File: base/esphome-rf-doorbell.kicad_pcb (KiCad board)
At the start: 2 copper layers, 65 x 54.7 mm, 100 parts, among them J1 B4B-XH, J2 CONUFL001-SMD-T, J3 Conn_01x01, J4 Conn_01x01, SW1 Boot, U1 BQ25628E, U2 RFM69W, U3 TPS7A2033, U4 MAX17261xxTD, U5 TPS629206DRLR, U6 G3VM-31DR, U7 ESP32-S2-MINI-2, U8 G3VM-63ER, U9 TLP2391

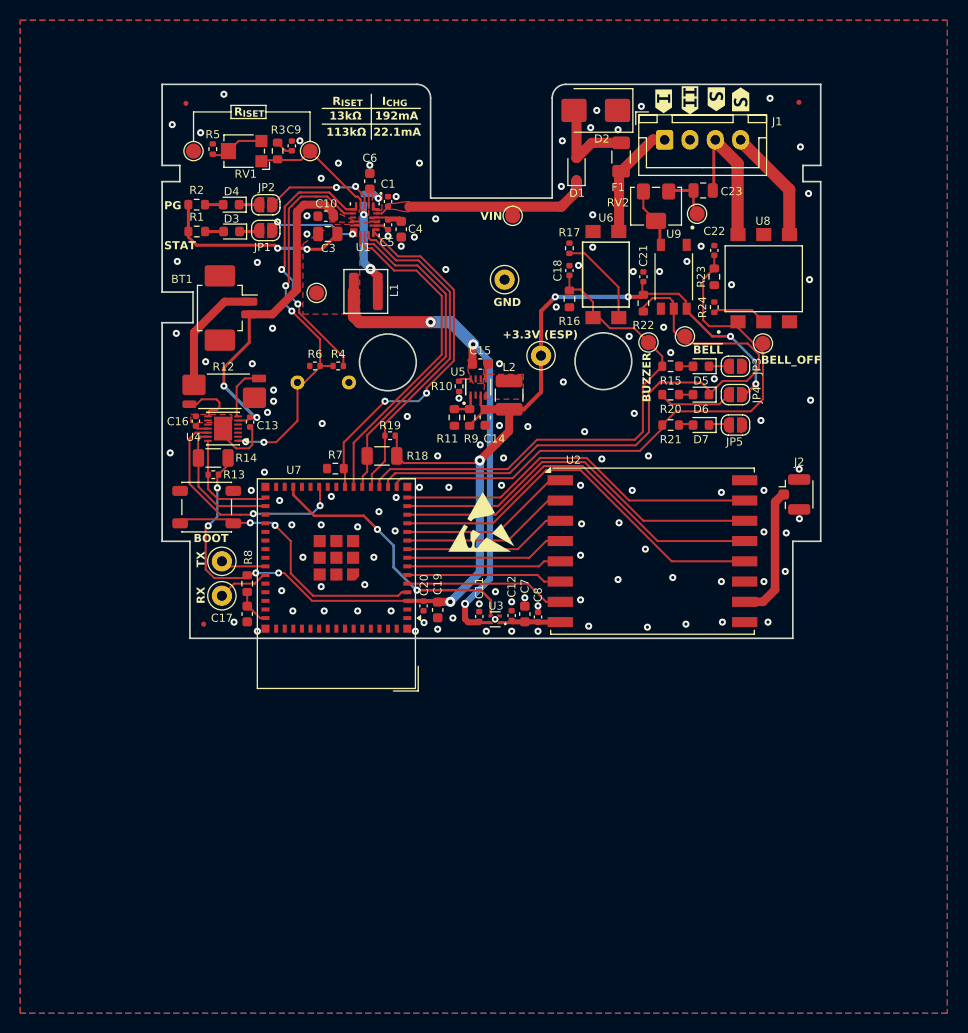
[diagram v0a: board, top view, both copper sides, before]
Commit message: Base board Rev3
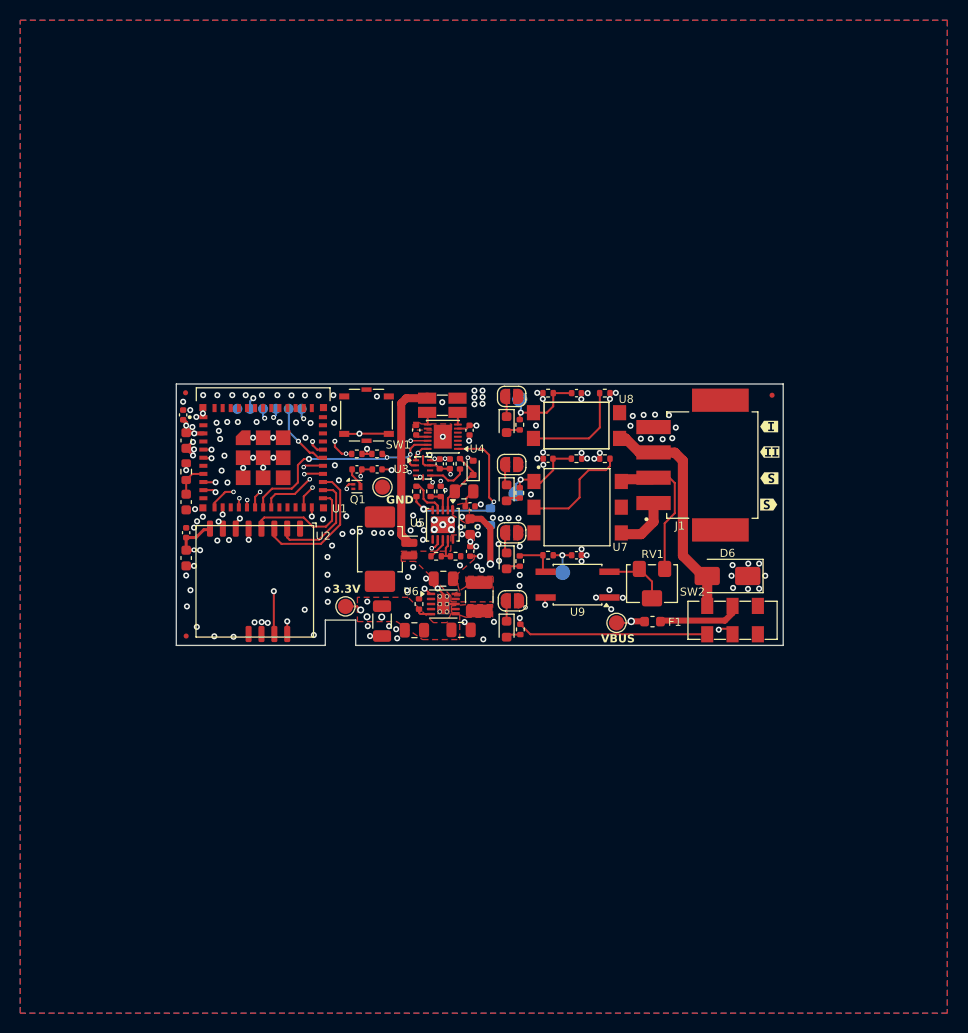
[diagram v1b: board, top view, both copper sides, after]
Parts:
- removed the C1 at (130.3, 77.9)
- removed the C2 at (127.9, 77.7)
- removed C21: 0.1uF, Capacitor_SMD:C_0402_1005Metric
- removed C23: 1uF 50V, Capacitor_SMD:C_0805_2012Metric
- removed the C3 at (124.3, 81.1)
- removed the C4 at (131.6, 80.6)
- removed the C5 at (130.3, 80.2)
- removed the D3 at (114.9, 80.8)
- removed the D4 at (114.8, 78.2)
- removed J3, J4: Conn_01x01, TestPoint:TestPoint_Keystone_5000-5004_Miniature
- removed the JP1 at (118.2, 80.8)
- removed the JP2 at (118.2, 78.2)
- removed L2: 2.2uH, Inductor_SMD:L_1210_3225Metric
- removed the R1 at (111.4, 80.8)
- removed the R10 at (137.3, 96.1)
- removed the R2 at (111.4, 78.2)
- removed the R20 at (158.2, 96.9)
- removed the R21 at (158.2, 99.9)
- removed the R4 at (125.4, 94.1)
- removed the REF** at (139.5, 109.5)
- removed the REF** at (117.4, 72.1)
- removed the RV1 at (116.0, 72.9)
- removed the TP1 at (122.6, 72.9)
- removed TP11: TestPoint, TestPoint:TestPoint_Pad_D1.5mm
- removed the TP4 at (123.2, 86.9)
- removed the TP5 at (111.1, 72.9)
- removed the U7 at (125.2, 115.6)
- removed kibuzzard-691E1EB0: G***, kibuzzard-691E1EB0
- removed kibuzzard-691E1EB7: G***, kibuzzard-691E1EB7
- removed kibuzzard-691E1ECB: G***, kibuzzard-691E1ECB
- removed kibuzzard-691E1ED6: G***, kibuzzard-691E1ED6
- added C16: 1uF, Capacitor_SMD:C_0402_1005Metric, F.Cu at (138.4, 112.4)
- added C19: 1uF, Capacitor_SMD:C_0402_1005Metric, F.Cu at (148.9, 112.8)
- added C8: 47uF, Capacitor_SMD:C_0805_2012Metric, F.Cu at (132.9, 120.2)
- added D5: Red, LED_SMD:LED_0603_1608Metric, F.Cu at (142.0, 120.1)
- added JP4: SolderJumper_2_Open, Jumper:SolderJumper-2_P1.3mm_Open_RoundedPad1.0x1.5mm, F.Cu at (142.6, 117.3)
- added Q1: PMZB390UNE, Package_DFN_QFN:Diodes_DFN1006-3, F.Cu at (127.2, 106.0)
- added R12: 1.27M, Resistor_SMD:R_0402_1005Metric, F.Cu at (137.0, 112.9)
- added R16: 1k, Resistor_SMD:R_0402_1005Metric, F.Cu at (143.3, 106.6)
- added R17: 1k, Resistor_SMD:R_0402_1005Metric, F.Cu at (143.3, 113.4)
- added R18: 1k, Resistor_SMD:R_0402_1005Metric, F.Cu at (143.4, 120.1)
- added R8: 47k, Resistor_SMD:R_0402_1005Metric, F.Cu at (134.5, 106.5)
- added REF**: KiCad-Logo2_6mm_SilkScreen, Symbol:KiCad-Logo2_6mm_SilkScreen, B.Cu at (118.7, 113.4)
- added SW2: CL-SB-22A-11T, lib:CL-SB-22A, F.Cu at (164.3, 119.2)
- added U6: TPS63900, Package_SON:WSON-10-1EP_2.5x2.5mm_P0.5mm_EP1.2x2mm_ThermalVias, F.Cu at (135.8, 117.6)
- added kibuzzard-696E5F1B: G***, kibuzzard-696E5F1B, F.Cu at (168.0, 102.6)
- added kibuzzard-696E5F26: G***, kibuzzard-696E5F26, F.Cu at (167.9, 100.1)
- added kibuzzard-696E5F32: G***, kibuzzard-696E5F32, F.Cu at (167.9, 105.2)
- added kibuzzard-696E5F3B: G***, kibuzzard-696E5F3B, F.Cu at (167.9, 107.8)
- C10: value 10uF 10V -> 47uF; footprint Capacitor_SMD:C_0603_1608Metric -> Capacitor_SMD:C_0805_2012Metric
- C12: value 1uF -> 47uF; footprint Capacitor_SMD:C_0402_1005Metric -> Capacitor_SMD:C_0805_2012Metric
- C14: value 22uF 6.3V -> 1uF 25V; footprint Capacitor_SMD:C_0603_1608Metric -> Capacitor_SMD:C_0402_1005Metric
- C15: value 4.7uF -> 10uF 25V
- C6: value 4.7uF -> 100uF; footprint Capacitor_SMD:C_0603_1608Metric -> Capacitor_SMD:C_1206_3216Metric
- C7: renamed from C16; value 47nF -> 0.47uF
- C9: value 330nF -> 0.1uF
- D1: value PMEG2005EJ-QX -> BAS70; footprint Diode_SMD:D_SOD-323F -> Diode_SMD:D_SOD-523
- D3: renamed from D7; value Red -> Blue
- D6: renamed from D2; value SMBJ15CA -> SMAJ15CA; footprint Diode_SMD:D_SMB -> Diode_SMD:D_SMA
- F1: value 250mA -> 80mA; footprint Fuse:Fuse_1206_3216Metric -> Fuse:Fuse_0603_1608Metric
- J1: value B4B-XH -> PTSM 0,5/ 4-2,5-H SMD R24; footprint Connector_JST:JST_XH_B4B-XH-A_1x04_P2.50mm_Vertical -> lib:PHOENIX_1702474
- J2: value CONUFL001-SMD-T -> Conn_01x06; footprint Connector_Coaxial:U.FL_Hirose_U.FL-R-SMT-1_Vertical -> lib:Connector_PogoClamp_1.27mm; moved to B.Cu
- L1: value 1.5uH -> 2.2uH; footprint Inductor_SMD:L_Wuerth_MAPI-4020 -> Inductor_SMD:L_1210_3225Metric
- R10: renamed from R12; value 25m -> 15m; footprint Resistor_SMD:R_Shunt_Vishay_WSK2512_6332Metric_T1.19mm -> lib:R_Shunt_D1WRL1206
- R11: value 137k -> 30k; footprint Resistor_SMD:R_0603_1608Metric -> Resistor_SMD:R_0402_1005Metric
- R13: value 4.7k -> 120k
- R14: value 4.7k -> 820k; footprint Resistor_SMD:R_1206_3216Metric -> Resistor_SMD:R_0805_2012Metric
- R15: footprint Resistor_SMD:R_0603_1608Metric -> Resistor_SMD:R_0402_1005Metric
- R19: renamed from R16; value 10k -> 100k; footprint Resistor_SMD:R_0603_1608Metric -> Resistor_SMD:R_0402_1005Metric
- R2: renamed from R18; value 4.7k -> 16.9k; footprint Resistor_SMD:R_1206_3216Metric -> Resistor_SMD:R_0402_1005Metric
- R20: renamed from R22; footprint Resistor_SMD:R_0603_1608Metric -> Resistor_SMD:R_0402_1005Metric
- R21: renamed from R23; value 10k -> 100k; footprint Resistor_SMD:R_0603_1608Metric -> Resistor_SMD:R_0402_1005Metric
- R3: value 1.2k -> 100k 0.1%; footprint Resistor_SMD:R_0603_1608Metric -> Capacitor_SMD:C_0402_1005Metric
- R4: renamed from R19; value 4.7k -> 16.9k
- R5: value 13k -> 1M 0.1%; footprint Resistor_SMD:R_0402_1005Metric -> Capacitor_SMD:C_0402_1005Metric
- R6: value 30.1k -> 10k
- R7: value 10k -> 16.2k; footprint Resistor_SMD:R_0603_1608Metric -> Resistor_SMD:R_0402_1005Metric
- R9: value 619k -> 499k; footprint Resistor_SMD:R_0603_1608Metric -> Resistor_SMD:R_0402_1005Metric
- SW1: value Boot -> Flash; footprint Button_Switch_SMD:SW_SPST_PTS647_Sx50 -> Button_Switch_SMD:SW_SPST_Panasonic_EVQPL_3PL_5PL_PT_A08
- TH1: footprint Resistor_THT:R_Axial_DIN0204_L3.6mm_D1.6mm_P5.08mm_Vertical -> Resistor_SMD:R_0603_1608Metric
- TP1: renamed from TP2; footprint TestPoint:TestPoint_Keystone_5000-5004_Miniature -> TestPoint:TestPoint_Pad_D1.5mm
- TP2: renamed from TP7; footprint TestPoint:TestPoint_Keystone_5000-5004_Miniature -> TestPoint:TestPoint_Pad_D1.5mm
- TP4: renamed from TP8; moved to B.Cu
- TP5: renamed from TP9; moved to B.Cu
- TP6: renamed from TP10; moved to B.Cu
- U1: value BQ25628E -> ESP32-C6-MINI-1; footprint lib:WQFN-HR18__RYK_TEX -> lib:XCVR_ESP32-C6-MINI-1U-N4
- U2: value RFM69W -> Wio-SX1262; footprint RF_Module:HOPERF_RFM69HW -> lib:Wio-SX1262 PCB Package
- U3: value TPS7A2033 -> ISL23315; footprint Package_SON:Texas_X2SON-4_1x1mm_P0.65mm -> lib:L10_2P1X1P6A_INR
- U4: value MAX17261xxTD -> MAX17260
- U5: value TPS629206DRLR -> LTC4079; footprint lib:SOT5X3-8_DRL_TEX -> Package_DFN_QFN:DFN-10-1EP_3x3mm_P0.5mm_EP1.65x2.38mm
- U9: value TLP2391 -> LTV-354T; footprint lib:OPTO_TLP2367_TPR_E -> Package_SO:SO-4_4.4x3.6mm_P2.54mm
- moved J2 52.5 mm to (118.6, 98.3), turned to 90 degrees
- moved D6 47.8 mm to (163.8, 114.8)
- moved F1 46.0 mm to (156.4, 119.3), turned to 180 degrees
- moved C6 43.4 mm to (129.7, 119.3), turned to -90 degrees
- moved TP3 41.5 mm to (152.8, 119.5)
- moved J1 38.5 mm to (166.8, 109.2), turned to 90 degrees
- moved C10 37.6 mm to (135.8, 115.1), turned to 180 degrees
- moved RV1 37.3 mm to (156.3, 115.6)
- moved REF** 36.1 mm to (118.7, 107.0)
- moved C4 35.7 mm to (110.4, 110.6)
- moved R5 35.5 mm to (129.2, 104.3), turned to 180 degrees
- moved C9 34.6 mm to (135.4, 103.8), turned to 90 degrees
- moved C5 33.9 mm to (110.4, 113.1), turned to -90 degrees
- moved U2 33.5 mm to (122.9, 109.9), turned to 180 degrees
- moved R3 32.4 mm to (127.2, 104.3), turned to 180 degrees
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- renumbered C20 to C1, C22 to C17, C19 to C2, C17 to C3, C8 to C4, C7 to C5, D5 to D2, D6 to D4, FID3 to FID2, FID2 to FID3, JP3 to JP1, JP5 to JP2, JP4 to JP3, R8 to R1, R17 to R22, R24 to R23, RV2 to RV1, TP6 to TP3, U8 to U7, U6 to U8
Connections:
- net /BAT- renamed -BATT
- C1 pad 1: +3.3VP -> +3.3V
- C10 pad 1: GND -> +BATT
- C10 pad 2: +BATT -> GND
- C11 pad 1: VBUS -> +3.3V
- C12 pad 1: +3.3VA -> +3.3V
- C14 pad 1: +3.3VP -> VBUS
- C2 pad 1: +3.3VP -> +3.3V
- C3 pad 1: Net-(U7-EN) -> Net-(U1-EN)
- C4 pad 1: +3.3VA -> +3.3V
- C5 pad 1: +3.3VA -> +3.3V
- C6 pad 1: Net-(U1-REGN) -> +3.3V
- C9 pad 1: GND -> +3.3V
- C9 pad 2: Net-(C9-Pad2) -> GND
- D1 pad 1: /VIN -> /CHG_EN
- D2 pad 2: Net-(D5-A) -> Net-(D2-A)
- D4 pad 1: /~{BELL_SIGNAL} -> Net-(D4-K)
- D6 pad 2: Net-(D1-A) -> /I
- F1 pad 1: /I -> Net-(F1-Pad1)
- F1 pad 2: Net-(D1-A) -> VBUS
- J1 pad 1: /I -> /S_OUT
- J1 pad 2: GND -> /S_IN
- J1 pad 3: /S_IN -> /I
- J1 pad 4: /S_OUT -> GND
- J2 pad 1: /RF.Antenna -> /UART_TX
- J2 pad 2: GND -> /UART_RX
- JP3 pad 1: Net-(JP4-A) -> Net-(D4-K)
- JP3 pad 2: +3.3VP -> GND
- L1 pad 1: /SW -> Net-(U6-LX1)
- L1 pad 2: VBUS -> Net-(U6-LX2)
- R1 pad 1: +3.3VP -> +3.3V
- R1 pad 2: Net-(U7-EN) -> Net-(U1-EN)
- R11 pad 1: Net-(U5-FB/VSET) -> Net-(U5-PROG)
- R13 pad 1: +3.3VP -> /CHG_EN
- R13 pad 2: /SCL2 -> Net-(U3-RW)
- R14 pad 1: +3.3VP -> VBUS
- R14 pad 2: /SDA2 -> /CHG_EN
- R15 pad 1: Net-(D5-A) -> /OPEN_BUZZER
- R15 pad 2: /OPEN_BUZZER -> Net-(D2-A)
- R2 pad 1: +3.3VP -> +3.3V
- R2 pad 2: /SDA1 -> /SCL
- R20 pad 1: +3.3VP -> Net-(R17-Pad1)
- R20 pad 2: /~{BELL_SIGNAL} -> /BELL_SIGNAL
- R3 pad 1: Net-(C9-Pad2) -> Net-(U1-IO0)
- R3 pad 2: Net-(U1-ILIM) -> Net-(Q1-D)
- R4 pad 1: +3.3VP -> +3.3V
- R4 pad 2: /SCL1 -> /SDA
- R5 pad 1: GND -> VBUS
- R5 pad 2: Net-(R5-Pad2) -> Net-(U1-IO0)
- R6 pad 1: GND -> Net-(U5-NTCBIAS)
- R7 pad 1: /~{CE} -> Net-(U6-CFG3)
- R9 pad 1: +3.3VP -> Net-(U5-FB)
- R9 pad 2: Net-(U5-FB/VSET) -> Net-(U5-FBG)
- RV1 pad 1: Net-(C23-Pad1) -> /S_IN
- RV1 pad 2: Net-(U9-K) -> Net-(RV1-Pad2)
- RV1 pad 3: Net-(U9-K) -> Net-(RV1-Pad2)
- SW1 pad 2: Net-(U7-IO0) -> Net-(U1-IO9)
- TP1 pad 1: +3.3VP -> +3.3V
- TP3 pad 1: /VIN -> VBUS
- TP4 pad 1: /~{BELL_SIGNAL} -> /BELL_SIGNAL
- U1 pad 1: /BTST -> GND
- U1 pad 10: Net-(JP1-A) -> /BELL_OFF
- U1 pad 11: /~{INT} -> GND
- U1 pad 12: /SDA1 -> Net-(U1-IO0)
- U1 pad 13: /SCL1 -> /V_{PROG}
- U1 pad 14: /~{CE} -> GND
- U1 pad 15: GND -> Net-(Q1-G)
- U1 pad 16: /SW -> Net-(D1-A)
- U1 pad 17: Net-(U1-PMID) -> /SCL
- U1 pad 18: /VIN -> /SDA
- U1 pad 2: Net-(U1-REGN) -> GND
- U1 pad 3: Net-(JP2-A) -> +3.3V
- U1 pad 4: Net-(U1-ILIM) -> unconnected-(U1-NC-Pad4)
- U1 pad 5: Net-(U1-TS_BIAS) -> /BAT_ALERT
- U1 pad 6: /TH -> /RF_DIO1
- U1 pad 8: +BATT -> Net-(U1-EN)
- U1 pad 9: VBUS -> /BELL_SIGNAL
- U2 pad 1: /RF.Reset -> unconnected-(U2-RF_SW1-Pad1)
- U2 pad 10: /RF.Antenna -> GND
- U2 pad 11: GND -> /RF_BUSY
- U2 pad 12: /RF.SCLK -> /RF_DIO1
- U2 pad 2: /RF.IO0 -> /SPI_MISO
- U2 pad 3: /RF.IO1 -> /SPI_MOSI
- U2 pad 4: /RF.IO2 -> /SPI_CLK
- U2 pad 5: /RF.IO3 -> /RF_RST
- U2 pad 6: /RF.IO4 -> /~{CS_RF}
- U2 pad 7: /RF.IO5 -> GND
- U2 pad 8: +3.3VA -> +3.3V
- U2 pad 9: GND -> unconnected-(U2-ANT-Pad9)
- U3 pad 1: +3.3VA -> /SCL
- U3 pad 2: GND -> /SDA
- U3 pad 3: /RF_PWR_EN -> GND
- U3 pad 4: VBUS -> GND
- U4 pad 13: /SDA2 -> /SDA
- U4 pad 14: /SCL2 -> /SCL
- U5 pad 1: Net-(U5-FB/VSET) -> VBUS
- U5 pad 2: unconnected-(U5-PG-Pad2) -> /CHG_EN
- U5 pad 3: +3.3VP -> Net-(U5-PROG)
- U5 pad 4: Net-(U5-SW) -> Net-(U5-NTCBIAS)
- U5 pad 5: GND -> /TH
- U5 pad 6: VBUS -> GND
- U5 pad 7: VBUS -> Net-(JP4-A)
- U5 pad 8: Net-(U5-MODE) -> Net-(U5-FBG)
- U9 pad 3: Net-(U9-K) -> Net-(R17-Pad1)
- U9 pad 4: GND -> +3.3V
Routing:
- net +3.3VP: track 118.3 -> 0.00 mm, vias 10 -> 0
- net +3.3V: track 0.00 -> 105.9 mm, vias 0 -> 15
- net /~{BELL_SIGNAL}: track 62.8 -> 0.00 mm
- net /BELL_SIGNAL: track 0.00 -> 47.6 mm, vias 0 -> 2
- net /RF.SCLK: track 39.1 -> 0.00 mm
- net /RF.MISO: track 38.3 -> 0.00 mm
- net /RF.MOSI: track 37.4 -> 0.00 mm
- net /RF.CE: track 36.6 -> 0.00 mm
- net /~{CE}: track 36.2 -> 0.00 mm, vias 2 -> 0
- net /DC_EN: track 0.00 -> 34.6 mm, vias 0 -> 2
- net /~{INT}: track 33.5 -> 0.00 mm
- net /SDA1: track 33.3 -> 0.00 mm
- net /SCL1: track 33.1 -> 0.00 mm
- net /SCL: track 0.00 -> 32.9 mm, vias 0 -> 5
- net VBUS: track 67.7 -> 36.9 mm, vias 5 -> 4
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- added copper zone on F.Cu, net +3.3V
- added copper zone on In2.Cu, net +3.3V
- added copper zone on In1.Cu, net GND
- added copper zone on In2.Cu, net GND
- added copper zone on F.Cu, net Net-(U6-LX1)
- added copper zone on F.Cu, net Net-(U6-LX2)
- removed copper zone on F.Cu, net /BTST
- removed copper zone on F.Cu, net /SW
- removed copper zone on F.Cu, net /VIN
- removed copper zone on F.Cu, net Net-(U5-SW)
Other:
- board size 65 x 54.7 mm -> 59.9 x 25.8 mm
- copper layers 2 -> 4
- board text added: "3.3V"
- board text added: "BELL"
- board text added: "RXD"
- board text added: "SCL"
- board text added: "SDA"
- board text added: "Smart doorbell with remote for Homeassistant https://github.com/usimd/esphome-rf-doorbell, Rev ${Revision}"
- board text added: "TXD"
- board text added: "VBUS"
- board text removed: "+3.3V (ESP)"
- board text removed: "113kΩ"
- board text removed: "13kΩ"
- board text removed: "192mA"
- board text removed: "22.1mA"
- board text removed: "BOOT"
- board text removed: "I_{CHG}"
- board text removed: "PG"
- board text removed: "RX"
- board text removed: "R_{ISET}"
- board text removed: "STAT"
- board text removed: "Smart doorbell for STR HT2001 with remote for Homeassistant https://github.com/usimd/esphome-rf-doorbell, Rev ${Revision}"
- board text removed: "TX"
- board text removed: "VIN"
- board text removed: "~{BELL}"
